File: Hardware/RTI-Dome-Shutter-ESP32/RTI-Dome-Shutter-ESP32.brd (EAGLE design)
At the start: 90.2 x 76.3 mm, 65 parts, among them IC1 REG1117FA-5.0_500, IC2 24LC64T-I/SN, IC8 REG1117-3.3V, J1 691313510003, J10 691313510002, J11 691313510002, J12 691313510002, J2 XT60PW-M, J3 691313510003, J4 691313510003, J6 691313510003, J7 691313510003, J8 691313510002, J9 691313510002, U1 ESP32-DEVKITC-32E

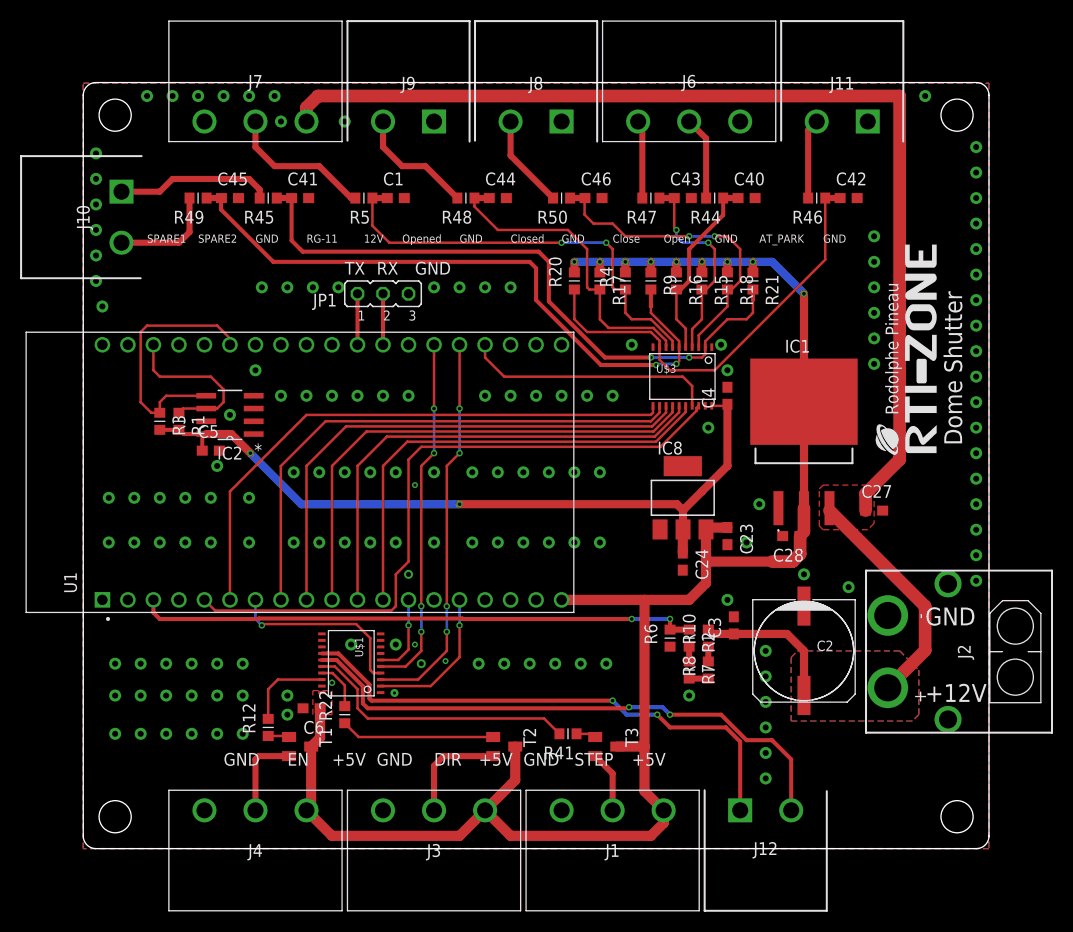
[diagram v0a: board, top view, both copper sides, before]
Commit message: Adding latest PCB files
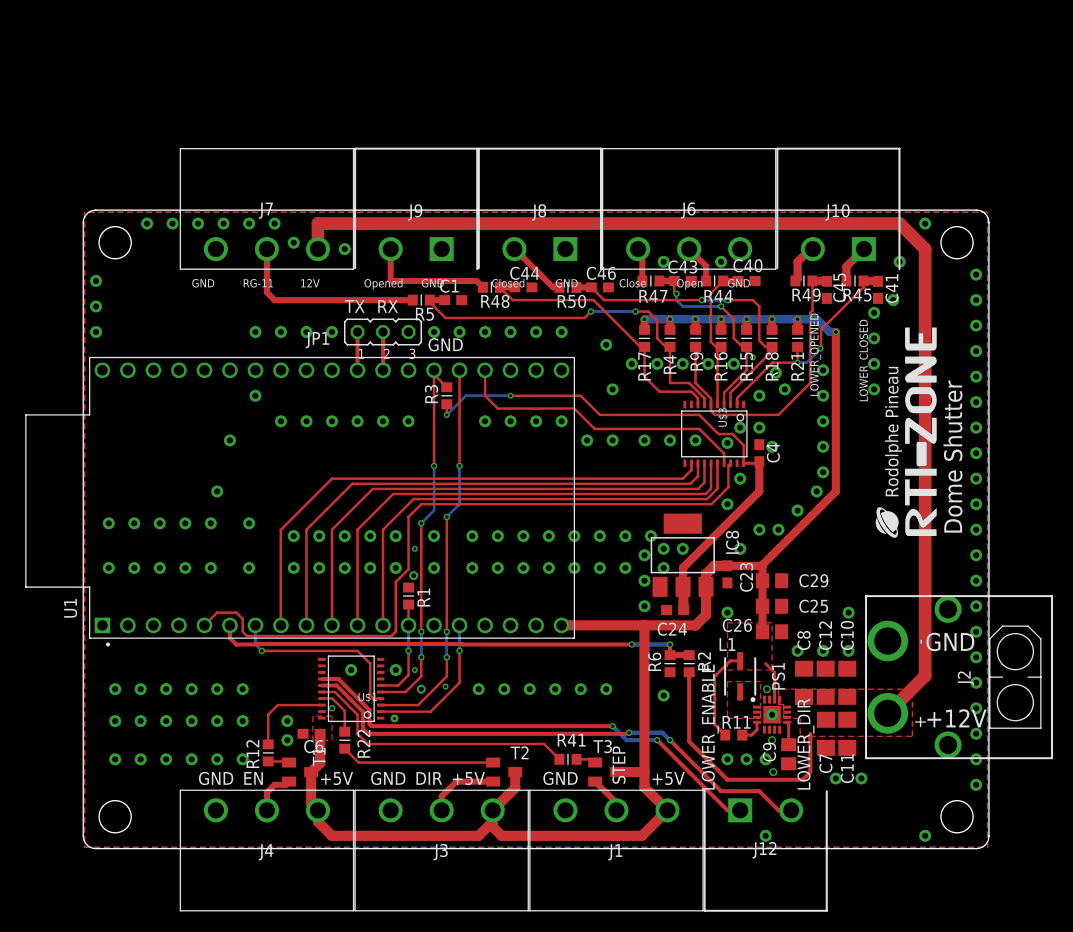
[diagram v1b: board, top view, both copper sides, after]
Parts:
- removed C2: 100uF, samacsys:UD-10X10_NICHICON
- removed C27, C28, C3, C42: 10uF, rti:C0603
- removed C5: 100nF, rti:C0603
- removed IC1: REG1117FA-5.0_500, REG1117FA-5.0_500:REG1117FA50500
- removed IC2: 24LC64T-I/SN, rti:SOIC127P600X175-8N
- removed J11: 691313510002, samacsys:SHDRRA2W100P0X508_1X2_1216X120
- removed R10, R7, R8: 100K 0.1%, rti:R0603
- removed R20: 4.7K, rti:R0603
- removed R46: 100, rti:R0603
- added C10, C11, C12: 22uF 35V, rcl:C1206
- added C25: 10uF, rcl:C0805
- added C26: 22uF, rcl:C0805
- added C29: 1uF, rcl:C0805
- added C7: 10uF, rcl:C1206
- added C8: 0.1uF, rcl:C1206
- added C9: 3.3nF, rcl:C0805
- added L1: IHLP1212BZER2R2M11, samacsys:INDPM3630X200N
- added PS1: TPS62133RGTR, samacsys:QFN50P300X300X100-17N
- added R11: 100K, rcl:R0603
- JP1: value (none) -> 3PIN_Header
- R1, R3: value 1K -> 100K
- R2: value 100K 0.1% -> 40K 0.1%
- R6: value 100K 0.1% -> 10K 0.1%
- T1, T2, T3: value (none) -> MMBT3904LT1
- moved J10 71.4 mm to (75.2, 59.7), turned to 180 degrees
- moved R49 60.9 mm to (71.8, 56.5)
- moved C45 60.1 mm to (74.0, 55.6), turned to 270 degrees
- moved R45 59.0 mm to (76.8, 56.5)
- moved C41 58.3 mm to (79.1, 55.6), turned to 270 degrees
- moved R1 28.7 mm to (32.4, 25.1)
- moved R3 28.7 mm to (36.2, 45.1), turned to 90 degrees
- moved J7 12.8 mm to (18.3, 59.7)
- moved J9 12.7 mm to (33.1, 59.7)
- moved J8 12.7 mm to (45.5, 59.7)
- moved J6 12.7 mm to (60.3, 59.7)
- moved C1 11.7 mm to (36.8, 54.6)
- moved R5 11.7 mm to (33.7, 54.6)
- moved C44 9.25 mm to (43.8, 55.9)
- moved R48 9.25 mm to (40.6, 55.9)
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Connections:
- net BUTTON_EAST_OPEN renamed BUTTON_OPEN
- net BUTTON_EAST_OPEN-IN_EXT renamed BUTTON_OPEN-IN_EXT
- net BUTTON_EAST_OPEN_5V renamed BUTTON_OPEN_5V
- net BUTTON_WEST_CLOSE renamed BUTTON_CLOSE
- net BUTTON_WEST_CLOSE-IN_EXT renamed BUTTON_CLOSE-IN_EXT
- net BUTTON_WEST_CLOSE_IN_5V renamed BUTTON_CLOSE_IN_5V
- net HOME_SHUTTER_CLOSED renamed SHUTTER_CLOSED
- net HOME_SHUTTER_CLOSED-IN_EXT renamed SHUTTER_CLOSED-IN_EXT
- net HOME_SHUTTER_CLOSED_IN_5V renamed SHUTTER_CLOSED_IN_5V
- net SPARE1 renamed LOWER_CLOSED
- net SPARE1-IN_EXT renamed LOWER_CLOSED-IN_EXT
- net SPARE1_IN_5V renamed LOWER_CLOSED_IN_5V
- net SPARE2 renamed LOWER_OPENED
- net SPARE2-IN_EXT renamed LOWER_OPENED-IN_EXT
- net SPARE2_IN_5V renamed LOWER_OPENED_IN_5V
- net SPARE_OUT1_5V renamed LOWER_DIR_5V
- net SPARE_OUT2_5V renamed LOWER_ENABLE_5V
- removed net AT_PARK_PIN: U$3.P$11, U1.6
- removed net AT_PARK_PIN-IN_EXT: J11.2, R46.2
- removed net AT_PARK_PIN_IN_5V: C42.1, R20.1, R46.1, U$3.P$9
- removed net N$2: R7.2, R8.1
- removed net N$3: R10.1, R8.2
- removed net N$5: R2.2, R7.1
- removed net SPARE_OUT1: U$1.P$5, U1.25
- removed net SPARE_OUT2: U$1.P$6, U1.13
- new net LOWER_DIR: R3.2, U$1.P$5, U1.25
- new net LOWER_ENABLE: R1.2, U$1.P$6, U1.13
- new net N$1: U$3.P$11
- new net PG: PS1.4, R11.2
- new net SS/TR: C9.1, PS1.9
- new net SW: L1.1, PS1.1, PS1.2, PS1.3
- net +12V: now also C10.1, C11.1, C12.1, C7.1, C8.1, PS1.10, PS1.11, PS1.12, PS1.13, R2.2; no longer C2.+, C27.1, C3.1, IC1.3, R10.2
- net 3.3V: now also R3.1; no longer C5.1, IC2.8, R1.2, R3.2
- net GND: now also C10.2, C11.2, C12.2, C25.1, C26.1, C29.1, C7.2, C8.2, C9.2, PS1.15, PS1.16, PS1.17, PS1.5, PS1.6, PS1.7, PS1.8, R1.1, U$3.P$9; no longer C2.-, C27.2, C28.2, C3.2, C42.2, C5.2, IC1.1, IC2.1, IC2.2, IC2.3, IC2.4, J11.1
- net SCL: no longer IC2.6, R1.1
- net SDA: no longer IC2.5, R3.1
- net VCC: now also C25.2, C26.2, C29.2, L1.2, PS1.14, R11.1; no longer C28.1, IC1.2, IC1.4, R20.2
- net VPIN: now also U1.6; no longer U1.3
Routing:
- net AT_PARK_PIN: track 56.8 -> 0.00 mm
- net AT_PARK_PIN_IN_5V: track 43.3 -> 0.00 mm
- net LOWER_CLOSED_IN_5V: track 63.7 -> 23.0 mm
- net LOWER_DIR: track 0.00 -> 37.9 mm, vias 0 -> 4
- net SPARE_OUT1: track 35.7 -> 0.00 mm, vias 4 -> 0
- net LOWER_OPENED_IN_5V: track 65.1 -> 30.1 mm, vias 2 -> 0
- net SDA: track 25.6 -> 0.00 mm
- net 3.3V: track 75.5 -> 54.8 mm
- net SCL: track 16.5 -> 0.00 mm
- net LOWER_CLOSED-IN_EXT: track 15.6 -> 3.90 mm
- net LOWER_ENABLE: track 0.00 -> 10.2 mm, vias 0 -> 1
- net SPARE_OUT2: track 8.16 -> 0.00 mm, vias 1 -> 0
- net AT_PARK_PIN-IN_EXT: track 7.97 -> 0.00 mm
- net VPIN: track 56.0 -> 48.3 mm
- net LOWER_OPENED-IN_EXT: track 10.6 -> 4.04 mm
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- added copper zone on layer 1, net SW
- removed copper zone on layer 16, net +12V
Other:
- board size 90.2 x 76.3 mm -> 90.2 x 63.6 mm
- board text added: "LOWER_CLOSED"
- board text added: "LOWER_DIR"
- board text added: "LOWER_ENABLE"
- board text added: "LOWER_OPENED"
- board text removed: "AT_PARK"
- board text removed: "SPARE1"
- board text removed: "SPARE2"
